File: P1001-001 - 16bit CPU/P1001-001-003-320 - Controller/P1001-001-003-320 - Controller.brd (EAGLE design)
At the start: 200 x 48 mm, 108 parts, among them IC1 74LS138D, IC10 74ALS00D, IC11 74ABT164D, IC12 74ABT164D, IC13 74ABT164D, IC14 74LS138D, IC15 74ABT164D, IC16 74ABT164D, IC17 74ABT164D, IC18 74ABT164D, IC19 74ABT164D, IC2 74LS157D, IC20 74ABT164D, IC3 74LS138D, IC4 74LS138D, IC5 74LS138D, IC6 74LS157D, IC7 74LS157D, IC8 74LS157D, IC9 74LS157D, J1 22-27-2041-04

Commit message: Add the control board
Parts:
- removed ALU_HIGH, ALU_LOW, A_OUT2, B_IN_LOW, B_OUT2, C_REG, RAN_IN_2, STACK: (no value), jumper:JP4
- removed A_CLEAR, B_CLEAR, D_IN, RAM_IN_LOW, X_SWAP: (no value), led:SFH482
- removed BACKBUS, FRONTBUS: (no value), con-harting-ml:ML16
- removed B_IN_HIGH, RAM_PC_OUT, RAN_IN_3: (no value), jumper:JP1
- removed D_REG, RAN_IN_1, X_REG: (no value), jumper:JP2W
- removed IC11, IC12, IC13, IC15, IC16, IC17, IC18, IC19, IC20: 74ABT164D, 74xx-us:SO14
- removed IC14: 74LS138D, 74xx-us:SO16
- removed IC2, IC6, IC7, IC8, IC9: 74LS157D, 74xx-us:SO16
- removed JP5: (no value), jumper:JP2
- removed U$2, U$3: SST39VF1602-70-4I-EKE, 16bit:TSOP48
- added ABC_CLEAR, B_IN_LOW1, HALT_RESEDT_NEXTINS, PC_MAR_IR_IN, RAM_STACK_IN: (no value), jumper:JP2W
- added ADD_HIGH, ADD_LOW, ADD_MID, BA_HIGH, BA_LOW, BB_HIGH, BB_LOW, BC_HIGH, BC_LOW: 74ABT164D, 74xx-us:SO14
- added ADD_SUB, B_IN_HIGH1, CLEAR_OUNS, EXTRA_1_2_PINS, EXTRA_3_4_PINS, EXTRA_5_6_PINS, INTERUPTS, PC_INC_DEC, RAM_IMT_OUT: (no value), jumper:JP1
- added A_CLEAR_LED, B_CLEAR_LED, D_CLEAR_LED, D_HIGH, D_IN_H, D_IN_L, D_LOW, EXTRA1, EXTRA2, EXTRA3, EXTRA4, EXTRA5, EXTRA6, EXTRA_OUT1, EXTRA_OUT2, EXTRA_OUT3, EXTRA_OUT4, INTERUPT_OUT, PAUSE_INERUPT, PC_DEC, PLAY_INTERUPT, RAM_IN_L, ROL, ROR, STEP1, STEP2, STEP3, STEP4: (no value), led:SFH482
- added A_OUT_PINS, B_OUT_PIMS, C_X_OC_STACK_OUT, D_OUT_PINS, EXTRA_OUT, IN_C_D_X, LOGIC_OP, SHIFT_ROLL, STACK_C, STEP_PINS: (no value), jumper:JP4
- added BANKA, BANKB, BANKC: SST39VF1602-70-4I-EKE, 16bit:TSOP48
- added IC21, IC22, IC23: 74LS138D, 74xx-us:SO16
- added IC27: MEGA8535-A, atmel:TQFP44
- added POWER_PINS, READ_WRITE: (no value), jumper:JP2
- added PULL_DOWN, R12, R13, R14: (no value), rcl:M0805
- added R10, R7, R8: (no value), resistor-bourns:SO16
- added RN2: (no value), resistor-dil:SOMC20
- added SV3: (no value), con-harting-ml:ML16
- added SV5: (no value), con-harting-ml:ML6
- added SW_PROD_1, SW_PROD_2, SW_PROD_3, SW_PROD_4, SW_PROD_5: 74LS157D, 74xx-us:SO16
- A_IN_LOW: device jumper:JP4 -> jumper:JP2W
- JP4: device jumper:JP1 -> jumper:JP3Q
- U$1: value SST39VF1602-70-4I-EKE -> 4-DIGIT-7-SEGMENT; device 16bit:TSOP48 -> ADAFRUIT:4-DIGIT-7-SEGMENT
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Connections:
- removed net A-CLEAR: A_CLEAR.K, A_IN_LOW.4, IC14.15
- removed net ADD: ADD.K, ALU_LOW.1, IC3.15
- removed net AND: ALU_HIGH.3, AND.K, IC3.9
- removed net A_HIGH: A_HIGH.K, A_OUT2.2, IC5.14
- removed net A_IN: A_IN.K, A_IN_LOW.3, IC14.14
- removed net A_IN_H_H: A_IN_H_H.K, A_IN_LOW.1, IC14.12
- removed net A_IN_H_L: A_IN_HIGH.1, A_IN_H_L.K, IC14.10
- removed net A_IN_L_H: A_IN_HIGH.2, A_IN_L_H.K, IC14.11
- removed net A_IN_L_L: A_IN_LOW.2, A_IN_L_L.K, IC14.13
- removed net A_LOW: A_LOW.K, A_OUT2.3, IC5.13
- removed net A_OUT: A_OUT.K, A_OUT2.4, IC5.12
- removed net A_SWAP: A_OUT2.1, A_SWAP.K, IC5.15
- removed net BUS0: BACKBUS.1, IC4.1, IC5.1
- removed net BUS1: BACKBUS.2, IC4.2, IC5.2
- removed net BUS10: BACKBUS.11, C_IN.K, C_REG.1
- removed net BUS11: BACKBUS.12, D_IN.K, D_REG.1
- removed net BUS12: BACKBUS.13, X_IN.K, X_REG.1
- removed net BUS13: BACKBUS.14, IR_IN.K, RAN_IN_3.2
- removed net BUS14: BACKBUS.15, MAR_IN.K, RAN_IN_3.1
- removed net BUS15: BACKBUS.16, PC_IN.K, RAN_IN_2.4
- removed net BUS16: FRONTBUS.1, RAM_IN_LOW.K, RAN_IN_2.3
- removed net BUS17: FRONTBUS.2, RAM_IN_H.K, RAN_IN_2.2
- removed net BUS18: FRONTBUS.3, IC3.1
- removed net BUS19: FRONTBUS.4, IC3.2
- removed net BUS2: BACKBUS.3, IC4.3, IC5.3
- removed net BUS20: FRONTBUS.5, IC3.3
- removed net BUS21: FRONTBUS.6, PC_INC.K, RAN_IN_2.1
- removed net BUS22: FRONTBUS.7, STACK.2, STACK_INC.K
- removed net BUS23: FRONTBUS.8, STACK.3, STACK_DEC.K
- removed net BUS24: C_INC.K, C_REG.2, FRONTBUS.9
- removed net BUS25: C_DEC.K, C_REG.3, FRONTBUS.10
- removed net BUS26: FRONTBUS.11, RAN_IN_1.3, RESET.K
- removed net BUS27: FRONTBUS.12, HALT.K, RAN_IN_1.2
- removed net BUS28: FRONTBUS.13, NEXT_INS.K, RAN_IN_1.1
- removed net BUS29: FRONTBUS.14, STACK.1, STACK_IN.K
- removed net BUS3: BACKBUS.4, IC4.4, IC5.4
- removed net BUS30: FRONTBUS.15
- removed net BUS31: FRONTBUS.16
- removed net BUS4: BACKBUS.5, IC14.1
- removed net BUS5: BACKBUS.6, IC14.2
- removed net BUS6: BACKBUS.7, IC14.3
- removed net BUS7: BACKBUS.8, IC1.1
- removed net BUS8: BACKBUS.9, IC1.2
- removed net BUS9: BACKBUS.10, IC1.3
- removed net B_CLEAR: B_CLEAR.K, B_IN_LOW.4, IC1.15
- removed net B_HIGH: B_HIGH.K, B_OUT2.2, IC5.10
- removed net B_IN: B_IN.K, B_IN_LOW.3, IC1.14
- removed net B_IN_H_H: B_IN_H_H.K, B_IN_LOW.1, IC1.12
- removed net B_IN_H_L: B_IN_HIGH.1, B_IN_H_L.K, IC1.10
- removed net B_IN_L_H: B_IN_HIGH.2, B_IN_L_H.K, IC1.11
- removed net B_IN_L_L: B_IN_LOW.2, B_IN_L_L.K, IC1.13
- removed net B_LOW: B_LOW.K, B_OUT2.3, IC5.9
- removed net B_OUT: B_OUT.K, B_OUT2.4, IC5.7
- removed net B_SWAP: B_OUT2.1, B_SWAP.K, IC5.11
- removed net HALT_LED: NEXT_INS.A, R3.13
- removed net NOT: ALU_HIGH.1, IC3.11, NOT.K
- removed net OR: ALU_HIGH.2, IC3.10, OR.K
- removed net PC_OUT: IC4.14, PC_OUT.K
- removed net RAM_OUT: IC4.9, RAM_OUT.K
- removed net SHL: ALU_LOW.3, IC3.13, SHL.K
- removed net SHR: ALU_LOW.4, IC3.12, SHR.K
- removed net SUB: ALU_LOW.2, IC3.14, SUB.K
- removed net XOR: ALU_HIGH.4, IC3.7, XOR.K
- new net A: IC27.37, RN2.20
- new net B: IC27.36, RN2.19
- new net BANKA_PROG: BANKA.11, JP4.5, R12.1
- new net BANKB_PROG: BANKB.11, JP4.3, R13.1
- new net BANKC_PROG: BANKC.11, JP4.1, R14.1
- new net C: IC27.35, RN2.18
- new net D: IC27.34, RN2.17
- new net DIG0: IC27.40, U$1.PIN14
- new net DIG1: IC27.41, U$1.PIN11
- new net DIG2: IC27.42, U$1.PIN10
- new net DIG3: IC27.43, U$1.PIN6
- new net DP: IC27.30, RN2.13
- new net E: IC27.33, RN2.16
- new net EXTERN_BUS0: IC27.9, R10.1, SV3.1
- new net EXTERN_BUS1: IC27.10, R10.9, SV3.2
- new net EXTERN_BUS10: IC27.21, R10.6, SV3.11
- new net EXTERN_BUS11: IC27.22, R10.14, SV3.12
- new net EXTERN_BUS12: IC27.23, R10.7, SV3.13
- new net EXTERN_BUS13: IC27.24, R10.15, SV3.14
- new net EXTERN_BUS14: IC27.25, R10.8, SV3.15
- new net EXTERN_BUS15: IC27.26, PULL_DOWN.1, SV3.16
- new net EXTERN_BUS2: IC27.11, R10.2, SV3.3
- new net EXTERN_BUS3: IC27.12, R10.10, SV3.4
- new net EXTERN_BUS4: IC27.13, R10.3, SV3.5
- new net EXTERN_BUS5: IC27.14, R10.11, SV3.6
- new net EXTERN_BUS6: IC27.15, R10.4, SV3.7
- new net EXTERN_BUS7: IC27.16, R10.12, SV3.8
- new net EXTERN_BUS8: IC27.19, R10.5, SV3.9
- new net EXTERN_BUS9: IC27.20, R10.13, SV3.10
- new net F: IC27.32, RN2.15
- new net G: IC27.31, RN2.14
- new net N$100: D_OUT.A, R3.14
- new net N$101: D_LOW.A, R3.13
- new net N$102: D_HIGH.A, R3.12
- new net N$103: D_SWAP.A, R3.11
- new net N$104: R3.10, X_OUT.A
- new net N$105: PC_OUT.A, R3.9
- new net N$106: IC5.15, RAM_IMT_OUT.1, RAM_OUT.K
- new net N$107: IC5.14, INTERUPT_OUT.K, RAM_IMT_OUT.2
- new net N$108: EXTRA_OUT.4, EXTRA_OUT1.K, IC5.13
- new net N$109: EXTRA_OUT.3, EXTRA_OUT2.K, IC5.12
- new net N$110: EXTRA_OUT.2, EXTRA_OUT3.K, IC5.11
- new net N$111: EXTRA_OUT.1, EXTRA_OUT4.K, IC5.10
- new net N$112: R2.1, STACK_OUT.A
- new net N$113: EXTRA_OUT4.A, R2.8
- new net N$114: EXTRA_OUT3.A, R2.7
- new net N$115: EXTRA_OUT2.A, R2.6
- new net N$116: EXTRA_OUT1.A, R2.5
- new net N$117: R2.2, RAM_OUT.A
- new net N$118: INTERUPT_OUT.A, R2.3
- new net N$119: IC27.1, SV5.3
- new net N$120: IC27.3, SV5.4
- new net N$121: IC27.2, SV5.6
- new net N$122: IC27.4, SV5.2
- new net N$123: RN2.1, U$1.PIN13
- new net N$124: RN2.2, U$1.PIN9
- new net N$125: RN2.3, U$1.PIN4
- new net N$126: RN2.4, U$1.PIN2
- new net N$127: RN2.5, U$1.PIN1
- new net N$128: RN2.6, U$1.PIN12
- new net N$129: RN2.7, U$1.PIN5
- new net N$130: RN2.8, U$1.PIN3
- new net N$131: R2.15, STEP1.A
- new net N$132: R2.14, STEP2.A
- new net N$133: R2.13, STEP3.A
- new net N$134: R2.12, STEP4.A
- new net N$37: BANKA.27, BANKA.46, BANKB.27, BANKB.46, BANKC.27, BANKC.46
- new net N$42: BANKA.28, BANKB.28, BANKC.28, READ_WRITE.2
- new net N$43: EXTRA5.A, R8.5
- new net N$63: IC1.13, SHIFT_ROLL.4, SHL.K
- new net N$64: IC1.12, SHIFT_ROLL.3, SHR.K
- new net N$65: IC1.11, ROL.K, SHIFT_ROLL.2
- new net N$66: IC1.10, ROR.K, SHIFT_ROLL.1
- new net N$67: NOT.A, R7.9
- new net N$68: AND.A, R7.10
- new net N$69: OR.A, R7.11
- new net N$70: R7.12, XOR.A
- new net N$71: IC23.7, LOGIC_OP.1, XOR.K
- new net N$72: IC23.9, LOGIC_OP.2, OR.K
- new net N$73: AND.K, IC23.10, LOGIC_OP.3
- new net N$74: IC23.11, LOGIC_OP.4, NOT.K
- new net N$75: A_OUT.K, A_OUT_PINS.1, IC3.15
- new net N$76: A_LOW.K, A_OUT_PINS.2, IC3.14
- new net N$77: A_HIGH.K, A_OUT_PINS.3, IC3.13
- new net N$78: A_OUT_PINS.4, A_SWAP.K, IC3.12
- new net N$79: B_OUT.K, B_OUT_PIMS.1, IC3.11
- new net N$80: B_LOW.K, B_OUT_PIMS.2, IC3.10
- new net N$81: B_HIGH.K, B_OUT_PIMS.3, IC3.9
- new net N$82: B_OUT_PIMS.4, B_SWAP.K, IC3.7
- new net N$83: D_OUT.K, D_OUT_PINS.1, IC4.14
- new net N$84: C_OUT.K, C_X_OC_STACK_OUT.4, IC4.15
- new net N$85: D_LOW.K, D_OUT_PINS.2, IC4.13
- new net N$86: D_HIGH.K, D_OUT_PINS.3, IC4.12
- new net N$87: D_OUT_PINS.4, D_SWAP.K, IC4.11
- new net N$88: C_X_OC_STACK_OUT.3, IC4.10, X_OUT.K
- new net N$89: C_X_OC_STACK_OUT.2, IC4.9, PC_OUT.K
- new net N$90: C_X_OC_STACK_OUT.1, IC4.7, STACK_OUT.K
- new net N$91: A_OUT.A, R3.1
- new net N$92: A_LOW.A, R3.2
- new net N$93: A_HIGH.A, R3.3
- new net N$94: A_SWAP.A, R3.4
- new net N$95: B_OUT.A, R3.5
- new net N$96: B_LOW.A, R3.6
- new net N$97: B_HIGH.A, R3.7
- new net N$98: B_SWAP.A, R3.8
- new net N$99: C_OUT.A, R3.15
- new net WRITE_ENABLE: BANKA.14, BANKB.14, BANKC.14, JP3.2
- net !CLEAR: now also BANKA.12, BANKB.12, BANKC.12, CLEAR_OUNS.1; no longer JP4.1
- net ADDR_BUS0: now also BANKA.25, BANKB.25, BANKC.25, SW_PROD_1.12; no longer IC7.12, U$1.25, U$2.25, U$3.25
- net ADDR_BUS1: now also BANKA.24, BANKB.24, BANKC.24, SW_PROD_1.9; no longer IC7.9, U$1.24, U$2.24, U$3.24
- net ADDR_BUS10: now also BANKA.6, BANKB.6, BANKC.6, SW_PROD_3.7; no longer IC2.7, U$1.6, U$2.6, U$3.6
- net ADDR_BUS11: now also BANKA.5, BANKB.5, BANKC.5, SW_PROD_3.4; no longer IC2.4, U$1.5, U$2.5, U$3.5
- net ADDR_BUS12: now also BANKA.4, BANKB.4, BANKC.4, SW_PROD_4.4; no longer IC8.4, U$1.4, U$2.4, U$3.4
- net ADDR_BUS13: now also BANKA.3, BANKB.3, BANKC.3, SW_PROD_4.7; no longer IC8.7, U$1.3, U$2.3, U$3.3
- net ADDR_BUS14: now also BANKA.2, BANKB.2, BANKC.2, SW_PROD_4.9; no longer IC8.9, U$1.2, U$2.2, U$3.2
- net ADDR_BUS15: now also BANKA.1, BANKB.1, BANKC.1, SW_PROD_4.12; no longer IC8.12, U$1.1, U$2.1, U$3.1
- net ADDR_BUS16: now also BANKA.48, BANKB.48, BANKC.48, SW_PROD_5.4; no longer IC9.4, U$1.48, U$2.48, U$3.48
- net ADDR_BUS17: now also BANKA.17, BANKB.17, BANKC.17, SW_PROD_5.7; no longer IC9.7, U$1.17, U$2.17, U$3.17
- net ADDR_BUS18: now also BANKA.16, BANKB.16, BANKC.16, SW_PROD_5.9; no longer IC9.9, U$1.16, U$2.16, U$3.16
- net ADDR_BUS19: now also BANKA.9, BANKB.9, BANKC.9, SW_PROD_5.12; no longer IC9.12, U$1.9, U$2.9, U$3.9
- net ADDR_BUS2: now also BANKA.23, BANKB.23, BANKC.23, SW_PROD_1.7; no longer IC7.7, U$1.23, U$2.23, U$3.23
- net ADDR_BUS3: now also BANKA.22, BANKB.22, BANKC.22, SW_PROD_1.4; no longer IC7.4, U$1.22, U$2.22, U$3.22
- net ADDR_BUS4: now also BANKA.21, BANKB.21, BANKC.21, SW_PROD_2.12; no longer IC6.12, U$1.21, U$2.21, U$3.21
- net ADDR_BUS5: now also BANKA.20, BANKB.20, BANKC.20, SW_PROD_2.9; no longer IC6.9, U$1.20, U$2.20, U$3.20
- net ADDR_BUS6: now also BANKA.19, BANKB.19, BANKC.19, SW_PROD_2.7; no longer IC6.7, U$1.19, U$2.19, U$3.19
- net ADDR_BUS7: now also BANKA.18, BANKB.18, BANKC.18, SW_PROD_2.4; no longer IC6.4, U$1.18, U$2.18, U$3.18
- net ADDR_BUS8: now also BANKA.8, BANKB.8, BANKC.8, SW_PROD_3.12; no longer IC2.12, U$1.8, U$2.8, U$3.8
- net ADDR_BUS9: now also BANKA.7, BANKB.7, BANKC.7, SW_PROD_3.9; no longer IC2.9, U$1.7, U$2.7, U$3.7
- net ADDR_SHIFT: now also ADD_LOW.1, ADD_LOW.2; no longer IC11.1, IC11.2
- net CLEAR: now also CLEAR_OUNS.2; no longer JP4.2
- net CLK: now also POWER_PINS.1; no longer JP5.1
- net DATAA0: now also BANKA.29, BA_LOW.3, IC3.1, IC4.1, IC5.1; no longer IC15.3, U$1.29
- net DATAA1: now also BANKA.31, BA_LOW.4, IC3.2, IC4.2, IC5.2; no longer IC15.4, U$1.31
- net DATAA10: now also BANKA.34, BA_HIGH.5, EXTRA6.K, EXTRA_5_6_PINS.2; no longer IC16.5, U$1.34
- net DATAA11: now also ABC_CLEAR.1, A_CLEAR_LED.K, BANKA.36, BA_HIGH.6; no longer IC16.6, U$1.36
- net DATAA12: now also ABC_CLEAR.2, BANKA.39, BA_HIGH.10, B_CLEAR_LED.K; no longer IC16.10, U$1.39
- net DATAA13: now also ABC_CLEAR.3, BANKA.41, BA_HIGH.11, D_CLEAR_LED.K; no longer IC16.11, U$1.41
- net DATAA14: now also BANKA.43, BA_HIGH.12, INTERUPTS.1, PAUSE_INERUPT.K; no longer IC16.12, U$1.43
- net DATAA15: now also BANKA.45, BA_HIGH.13, INTERUPTS.2, PLAY_INTERUPT.K; no longer IC16.13, U$1.45
- net DATAA2: now also BANKA.33, BA_LOW.5, IC3.3, IC4.3, IC5.3; no longer IC15.5, U$1.33
- net DATAA3: now also BANKA.35, BA_LOW.6, IC3.4, IC4.4, IC5.4; no longer IC15.6, U$1.35
- net DATAA4: now also BANKA.38, BA_LOW.10, IC3.5, IC4.5, IC5.5; no longer IC15.10, U$1.38
- net DATAA5: now also BANKA.40, BA_LOW.11, EXTRA1.K, EXTRA_1_2_PINS.1; no longer IC15.11, U$1.40
- net DATAA6: now also BANKA.42, BA_LOW.12, EXTRA2.K, EXTRA_1_2_PINS.2; no longer IC15.12, U$1.42
- net DATAA7: now also BANKA.44, BA_HIGH.1, BA_HIGH.2, BA_LOW.13, EXTRA3.K, EXTRA_3_4_PINS.1; no longer IC15.13, IC16.1, IC16.2, U$1.44
- net DATAA8: now also BANKA.30, BA_HIGH.3, EXTRA4.K, EXTRA_3_4_PINS.2; no longer IC16.3, U$1.30
- net DATAA9: now also BANKA.32, BA_HIGH.4, EXTRA5.K, EXTRA_5_6_PINS.1; no longer IC16.4, U$1.32
- net DATAA_SHIFT: now also BA_LOW.1, BA_LOW.2; no longer IC15.1, IC15.2
- net DATAB0: now also BANKB.29, BB_LOW.3, IC21.1; no longer IC17.3, U$2.29
- net DATAB1: now also BANKB.31, BB_LOW.4, IC21.2; no longer IC17.4, U$2.31
- net DATAB10: now also BANKB.34, BB_HIGH.5, IR_IN.K, PC_MAR_IR_IN.1; no longer IC18.5, U$2.34
- net DATAB11: now also BANKB.36, BB_HIGH.6, MAR_IN.K, PC_MAR_IR_IN.2; no longer IC18.6, U$2.36
- net DATAB12: now also BANKB.39, BB_HIGH.10, PC_IN.K, PC_MAR_IR_IN.3; no longer IC18.10, U$2.39
- net DATAB13: now also BANKB.41, BB_HIGH.11, RAM_STACK_IN.1, STACK_IN.K; no longer IC18.11, U$2.41
- net DATAB14: now also BANKB.43, BB_HIGH.12, RAM_IN_L.K, RAM_STACK_IN.2; no longer IC18.12, U$2.43
- net DATAB15: now also BANKB.45, BB_HIGH.13, RAM_IN_H.K, RAM_STACK_IN.3; no longer IC18.13, U$2.45
- net DATAB2: now also BANKB.33, BB_LOW.5, IC21.3; no longer IC17.5, U$2.33
- net DATAB3: now also BANKB.35, BB_LOW.6, IC22.1; no longer IC17.6, U$2.35
- net DATAB4: now also BANKB.38, BB_LOW.10, IC22.2, PC_INC_DEC.2; no longer IC17.10, U$2.38
- net DATAB5: now also BANKB.40, BB_LOW.11, IC22.3; no longer IC17.11, U$2.40
- net DATAB6: now also BANKB.42, BB_LOW.12, C_IN.K, IN_C_D_X.1; no longer IC17.12, U$2.42
- net DATAB7: now also BANKB.44, BB_HIGH.1, BB_HIGH.2, BB_LOW.13, D_IN_L.K, IN_C_D_X.2; no longer IC17.13, IC18.1, IC18.2, U$2.44
- net DATAB8: now also BANKB.30, BB_HIGH.3, D_IN_H.K, IN_C_D_X.3; no longer IC18.3, U$2.30
- net DATAB9: now also BANKB.32, BB_HIGH.4, IN_C_D_X.4, X_IN.K; no longer IC18.4, U$2.32
- net DATAB_SHIFT: now also BB_LOW.1, BB_LOW.2; no longer IC17.1, IC17.2
- net DATAC0: now also BANKC.29, BC_LOW.3, IC1.1, IC23.1; no longer IC19.3, U$3.29
- net DATAC1: now also BANKC.31, BC_LOW.4, IC1.2, IC23.2; no longer IC19.4, U$3.31
- net DATAC10: now also BANKC.34, BC_HIGH.5; no longer IC20.5, U$3.34
- net DATAC11: now also BANKC.36, BC_HIGH.6; no longer IC20.6, U$3.36
- net DATAC12: now also BANKC.39, BC_HIGH.10; no longer IC20.10, U$3.39
- net DATAC13: now also BANKC.41, BC_HIGH.11, HALT_RESEDT_NEXTINS.3, RESET.K; no longer IC20.11, U$3.41
- net DATAC14: now also BANKC.43, BC_HIGH.12, HALT.K, HALT_RESEDT_NEXTINS.2; no longer IC20.12, U$3.43
- net DATAC15: now also BANKC.45, BC_HIGH.13, HALT_RESEDT_NEXTINS.1, NEXT_INS.K; no longer IC20.13, U$3.45
- net DATAC2: now also BANKC.33, BC_LOW.5, IC1.3, IC23.3; no longer IC19.5, U$3.33
- net DATAC3: now also BANKC.35, BC_LOW.6, IC1.4, IC23.4; no longer IC19.6, U$3.35
- net DATAC4: now also BANKC.38, BC_LOW.10, PC_DEC.K; no longer IC19.10, U$3.38
- net DATAC5: now also BANKC.40, BC_LOW.11, PC_INC.K, PC_INC_DEC.1; no longer IC19.11, U$3.40
- net DATAC6: now also BANKC.42, BC_LOW.12, STACK_C.4, STACK_INC.K; no longer IC19.12, U$3.42
- net DATAC7: now also BANKC.44, BC_HIGH.1, BC_HIGH.2, BC_LOW.13, STACK_C.3, STACK_DEC.K; no longer IC19.13, IC20.1, IC20.2, U$3.44
- net DATAC8: now also BANKC.30, BC_HIGH.3, C_INC.K, STACK_C.2; no longer IC20.3, U$3.30
- net DATAC9: now also BANKC.32, BC_HIGH.4, C_DEC.K, STACK_C.1; no longer IC20.4, U$3.32
- net DATAC_SHIFT: now also BC_LOW.1, BC_LOW.2; no longer IC19.1, IC19.2
- net DATA_ADDR_CLOCK: now also BA_HIGH.8, BA_LOW.8, BB_HIGH.8, BB_LOW.8, BC_HIGH.8, BC_LOW.8; no longer IC15.8, IC16.8, IC17.8, IC18.8, IC19.8, IC20.8
- net GND: now also ADD_HIGH.7, ADD_LOW.7, ADD_MID.7, BANKA.26, BANKA.37, BANKB.26, BANKB.37, BANKC.26, BANKC.37, BA_HIGH.7, BA_LOW.7, BB_HIGH.7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; no longer IC1.4, IC11.7, IC12.7, IC13.7, IC14.4, IC14.5, IC14.8, IC15.7, IC16.7, IC17.7, IC18.7, IC19.7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
- net IN_BUS0: now also STEP1.K, STEP_PINS.1, SW_PROD_1.14; no longer IC7.14
- net IN_BUS1: now also STEP2.K, STEP_PINS.2, SW_PROD_1.11; no longer IC7.11
- net IN_BUS10: now also SW_PROD_3.5; no longer IC2.5
- net IN_BUS11: now also SW_PROD_3.2; no longer IC2.2
- net IN_BUS12: now also SW_PROD_4.2; no longer IC8.2
- net IN_BUS13: now also SW_PROD_4.5; no longer IC8.5
- net IN_BUS14: now also SW_PROD_4.11; no longer IC8.11
- net IN_BUS15: now also SW_PROD_4.14; no longer IC8.14
- net IN_BUS16: now also SW_PROD_5.2; no longer IC9.2
- net IN_BUS17: now also SW_PROD_5.5; no longer IC9.5
- net IN_BUS18: now also SW_PROD_5.11; no longer IC9.11
- net IN_BUS19: now also SW_PROD_5.14; no longer IC9.14
- net IN_BUS2: now also STEP3.K, STEP_PINS.3, SW_PROD_1.5; no longer IC7.5
- net IN_BUS3: now also STEP4.K, STEP_PINS.4, SW_PROD_1.2; no longer IC7.2
- net IN_BUS4: now also SW_PROD_2.14; no longer IC6.14
- net IN_BUS5: now also SW_PROD_2.11; no longer IC6.11
- net IN_BUS6: now also SW_PROD_2.5; no longer IC6.5
- net IN_BUS7: now also SW_PROD_2.2; no longer IC6.2
- net IN_BUS8: now also SW_PROD_3.14; no longer IC2.14
- net IN_BUS9: now also SW_PROD_3.11; no longer IC2.11
- net N$10: now also D_CLEAR_LED.A, R8.9; no longer IC4.11, X_REG.2, X_SWAP.K
- net N$11: now also PAUSE_INERUPT.A, R8.10; no longer R3.2, X_IN.A
- net N$12: now also PLAY_INTERUPT.A, R8.11; no longer IC4.7, X_OUT.K, X_REG.3
- net N$13: now also C_IN.A, R8.12; no longer R3.15, X_OUT.A
- net N$14: now also D_IN_L.A, R8.15; no longer R3.9, STACK_IN.A
- net N$15: now also D_IN_H.A, R8.14; no longer R3.10, STACK_INC.A
- net N$16: now also PC_INC.A, R5.1; no longer R3.11, STACK_DEC.A
- net N$17: now also PC_DEC.A, R5.2; no longer R3.12, STACK_OUT.A
- net N$18: now also IR_IN.A, R5.3; no longer IC4.13, STACK.4, STACK_OUT.K
- net N$19: now also MAR_IN.A, R5.4; no longer D_REG.2, D_SWAP.K, IC4.15
- net N$2: now also EXTRA1.A, R8.1; no longer C_IN.A, R3.8
- net N$20: now also PC_IN.A, R5.5; no longer D_SWAP.A, R3.14
- net N$21: now also R5.6, STACK_IN.A; no longer A_CLEAR.A, R5.9
- net N$22: now also R5.7, RAM_IN_L.A; no longer ADD.A, R5.1
- net N$23: now also R5.8, RAM_IN_H.A; no longer A_IN.A, R5.10
- net N$24: now also NEXT_INS.A, R5.10; no longer B_CLEAR.A, R4.9
- net N$25: now also R5.15, STACK_DEC.A; no longer B_IN.A, R4.10
- net N$26: now also C_INC.A, R5.14; no longer B_IN_L_L.A, R4.11
- net N$27: now also C_DEC.A, R5.13; no longer B_IN_H_H.A, R4.12
- net N$28: now also R5.12, RESET.A; no longer R5.8, XOR.A
- net N$29: now also HALT.A, R5.11; no longer AND.A, R5.7
- net N$3: now also EXTRA2.A, R8.2; no longer C_OUT.K, C_REG.4, IC4.10
- net N$30: now also R5.9, STACK_INC.A; no longer OR.A, R5.6
- net N$31: now also A_IN.K, A_IN_LOW.1, IC21.15; no longer NOT.A, R5.5
- net N$32: now also A_IN_LOW.2, A_IN_L_L.K, IC21.14; no longer R5.4, SHR.A
- net N$33: now also A_IN_H_H.K, A_IN_LOW.3, IC21.13; no longer R5.3, SHL.A
- net N$34: now also A_IN_HIGH.1, A_IN_L_H.K, IC21.12; no longer R5.2, SUB.A
- net N$35: now also A_IN_HIGH.2, A_IN_H_L.K, IC21.11; no longer B_IN_L_H.A, R4.13
- net N$36: now also A_IN.A, R4.8; no longer B_IN_H_L.A, R4.14
- net N$38: now also R4.7; no longer R5.11
- net N$39: now also R4.6; no longer R5.12
- net N$4: now also R8.13, X_IN.A; no longer C_OUT.A, R3.5
- net N$40: now also R4.5; no longer R5.13
- net N$41: now also R4.4; no longer R5.14
- net N$44: now also B_IN.A, B_IN_LOW1.3, IC22.15; no longer R2.15, RAM_OUT.A, RAM_PC_OUT.2
- net N$45: now also B_IN_LOW1.2, B_IN_L_L.A, IC22.14; no longer A_SWAP.A, R2.1
- net N$46: now also B_IN_H_H.A, B_IN_LOW1.1, IC22.13; no longer A_HIGH.A, R2.2
- net N$47: now also B_IN_HIGH1.2, B_IN_L_H.A, IC22.12; no longer A_LOW.A, R2.3
- net N$48: now also B_IN_HIGH1.1, B_IN_H_L.A, IC22.11; no longer A_OUT.A, R2.4
- net N$49: now also B_IN.K, R4.9; no longer B_SWAP.A, R2.5
- net N$5: now also EXTRA4.A, R8.4; no longer C_DEC.A, R3.6
- net N$51: now also B_IN_L_L.K, R4.10; no longer B_HIGH.A, R2.6
- net N$52: now also B_IN_H_H.K, R4.11; no longer B_LOW.A, R2.7
- net N$53: now also B_IN_L_H.K, R4.12; no longer B_OUT.A, R2.8
- net N$54: now also B_IN_H_L.K, R4.14; no longer PC_OUT.A, R2.14, RAM_PC_OUT.1
- net N$55: now also R7.8, ROR.A; no longer IR_IN.A, R4.8
- net N$56: now also R7.7, ROL.A; no longer MAR_IN.A, R4.7
- net N$57: now also R7.6, SHR.A; no longer PC_IN.A, R4.6
- net N$58: now also R7.5, SHL.A; no longer R4.5, RAM_IN_LOW.A
- net N$59: now also R7.4, SUB.A; no longer R4.4, RAM_IN_H.A
- net N$6: now also EXTRA3.A, R8.3; no longer C_INC.A, R3.7
- net N$60: now also ADD.A, R7.3; no longer PC_INC.A, R4.3
- net N$61: now also ADD.K, ADD_SUB.2, IC1.15; no longer R4.2, RESET.A
- net N$62: now also ADD_SUB.1, IC1.14, SUB.K; no longer HALT.A, R4.1
- net N$7: now also EXTRA6.A, R8.6; no longer D_OUT.A, D_OUT.K, D_REG.3, IC4.12, R3.3
- net N$8: now also B_CLEAR_LED.A, R8.8; no longer D_IN.A, R3.4
- net N$9: now also A_CLEAR_LED.A, R8.7; no longer R3.1, X_SWAP.A
- net PROGRAM: now also JP4.2, JP4.4, JP4.6
- net PROG_ADDR0: now also ADD_LOW.3, SW_PROD_1.13; no longer IC11.3, IC7.13
- net PROG_ADDR1: now also ADD_LOW.4, SW_PROD_1.10; no longer IC11.4, IC7.10
- net PROG_ADDR10: now also ADD_MID.5, SW_PROD_3.6; no longer IC12.5, IC2.6
- net PROG_ADDR11: now also ADD_MID.6, SW_PROD_3.3; no longer IC12.6, IC2.3
- net PROG_ADDR12: now also ADD_MID.10, SW_PROD_4.3; no longer IC12.10, IC8.3
- net PROG_ADDR13: now also ADD_MID.11, SW_PROD_4.6; no longer IC12.11, IC8.6
- net PROG_ADDR14: now also ADD_MID.12, SW_PROD_4.10; no longer IC12.12, IC8.10
- net PROG_ADDR15: now also ADD_HIGH.1, ADD_HIGH.2, ADD_MID.13, SW_PROD_4.13; no longer IC12.13, IC13.1, IC13.2, IC8.13
- net PROG_ADDR16: now also ADD_HIGH.3, SW_PROD_5.3; no longer IC13.3, IC9.3
- net PROG_ADDR17: now also ADD_HIGH.4, SW_PROD_5.6; no longer IC13.4, IC9.6
- net PROG_ADDR18: now also ADD_HIGH.5, SW_PROD_5.10; no longer IC13.5, IC9.10
- net PROG_ADDR19: now also ADD_HIGH.6, SW_PROD_5.13; no longer IC13.6, IC9.13
- net PROG_ADDR2: now also ADD_LOW.5, SW_PROD_1.6; no longer IC11.5, IC7.6
- net PROG_ADDR3: now also ADD_LOW.6, SW_PROD_1.3; no longer IC11.6, IC7.3
- net PROG_ADDR4: now also ADD_LOW.10, SW_PROD_2.13; no longer IC11.10, IC6.13
- net PROG_ADDR5: now also ADD_LOW.11, SW_PROD_2.10; no longer IC11.11, IC6.10
- net PROG_ADDR6: now also ADD_LOW.12, SW_PROD_2.6; no longer IC11.12, IC6.6
- net PROG_ADDR7: now also ADD_LOW.13, ADD_MID.1, ADD_MID.2, SW_PROD_2.3; no longer IC11.13, IC12.1, IC12.2, IC6.3
- net PROG_ADDR8: now also ADD_MID.3, SW_PROD_3.13; no longer IC12.3, IC2.13
- net PROG_ADDR9: now also ADD_MID.4, SW_PROD_3.10; no longer IC12.4, IC2.10
- net PROG_ADDR_CLOCK: now also ADD_HIGH.8, ADD_LOW.8, ADD_MID.8; no longer IC11.8, IC12.8, IC13.8
- net PROG_CLEAR: now also ADD_HIGH.9, ADD_LOW.9, ADD_MID.9, BA_HIGH.9, BA_LOW.9, BB_HIGH.9, BB_LOW.9, BC_HIGH.9, BC_LOW.9; no longer IC11.9, IC12.9, IC13.9, IC15.9, IC16.9, IC17.9, IC18.9, IC19.9, IC20.9
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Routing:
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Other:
- board size 200 x 48 mm -> 200 x 152 mm

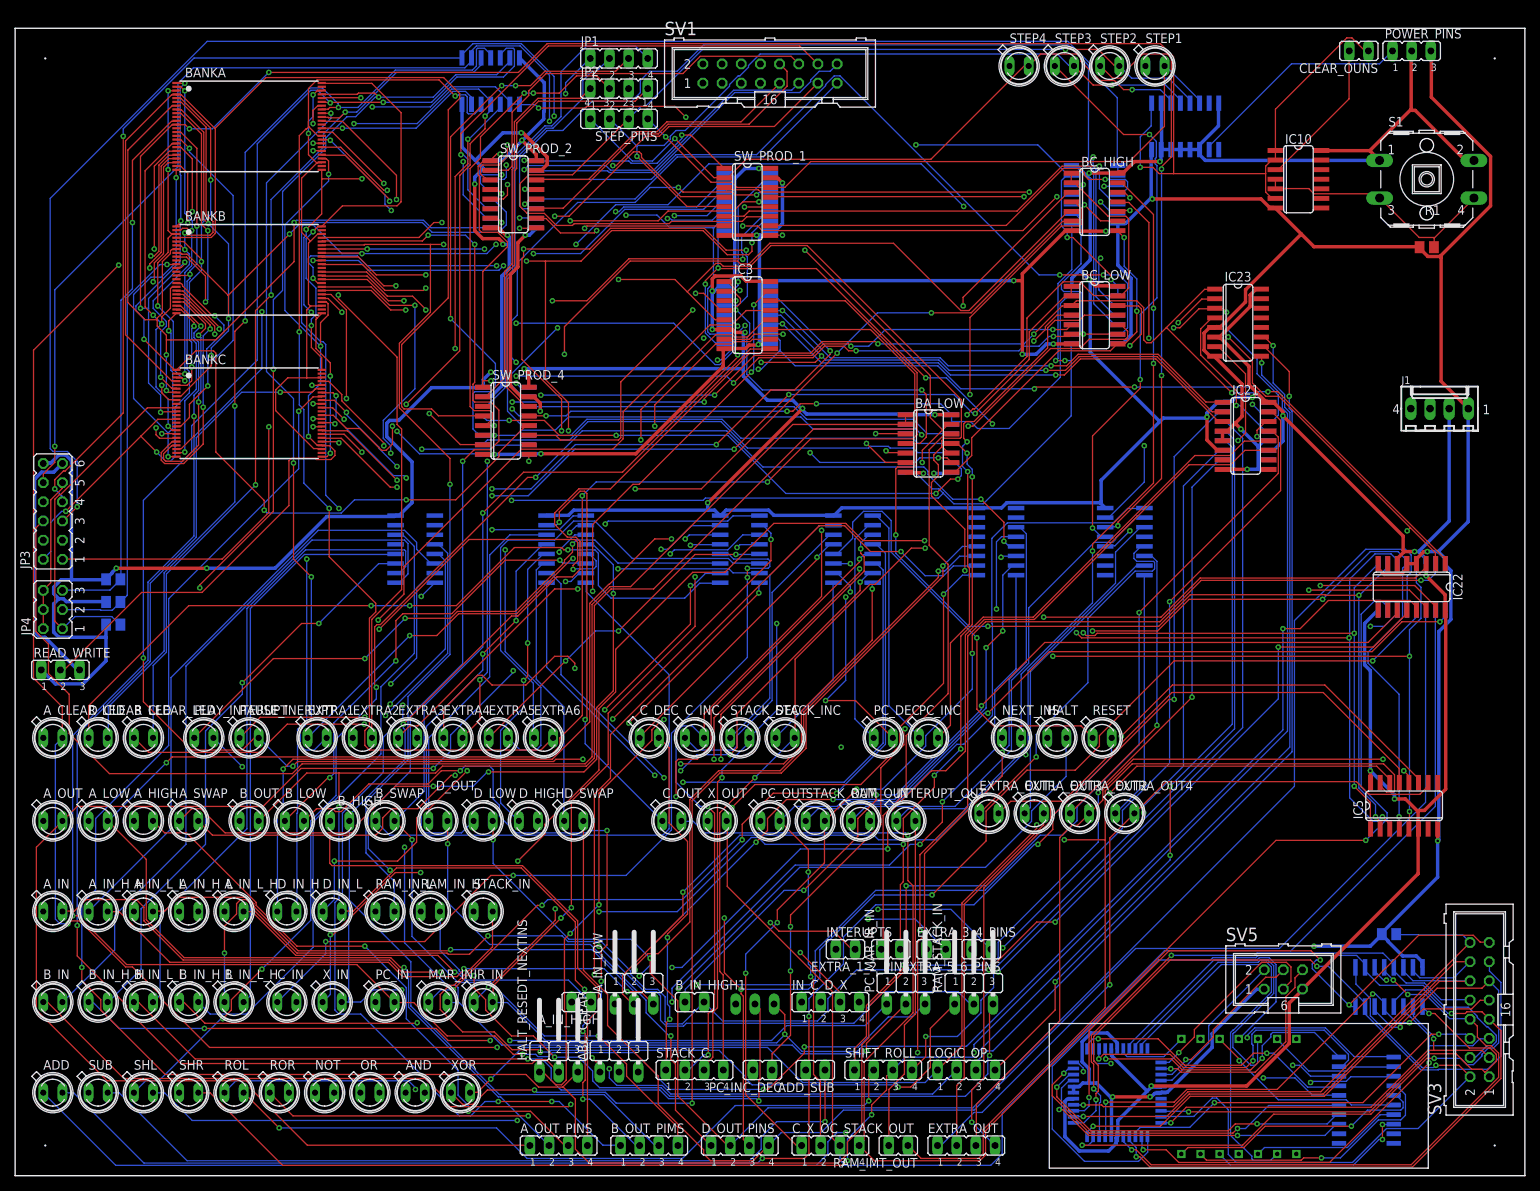
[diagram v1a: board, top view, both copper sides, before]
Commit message: Controller done?
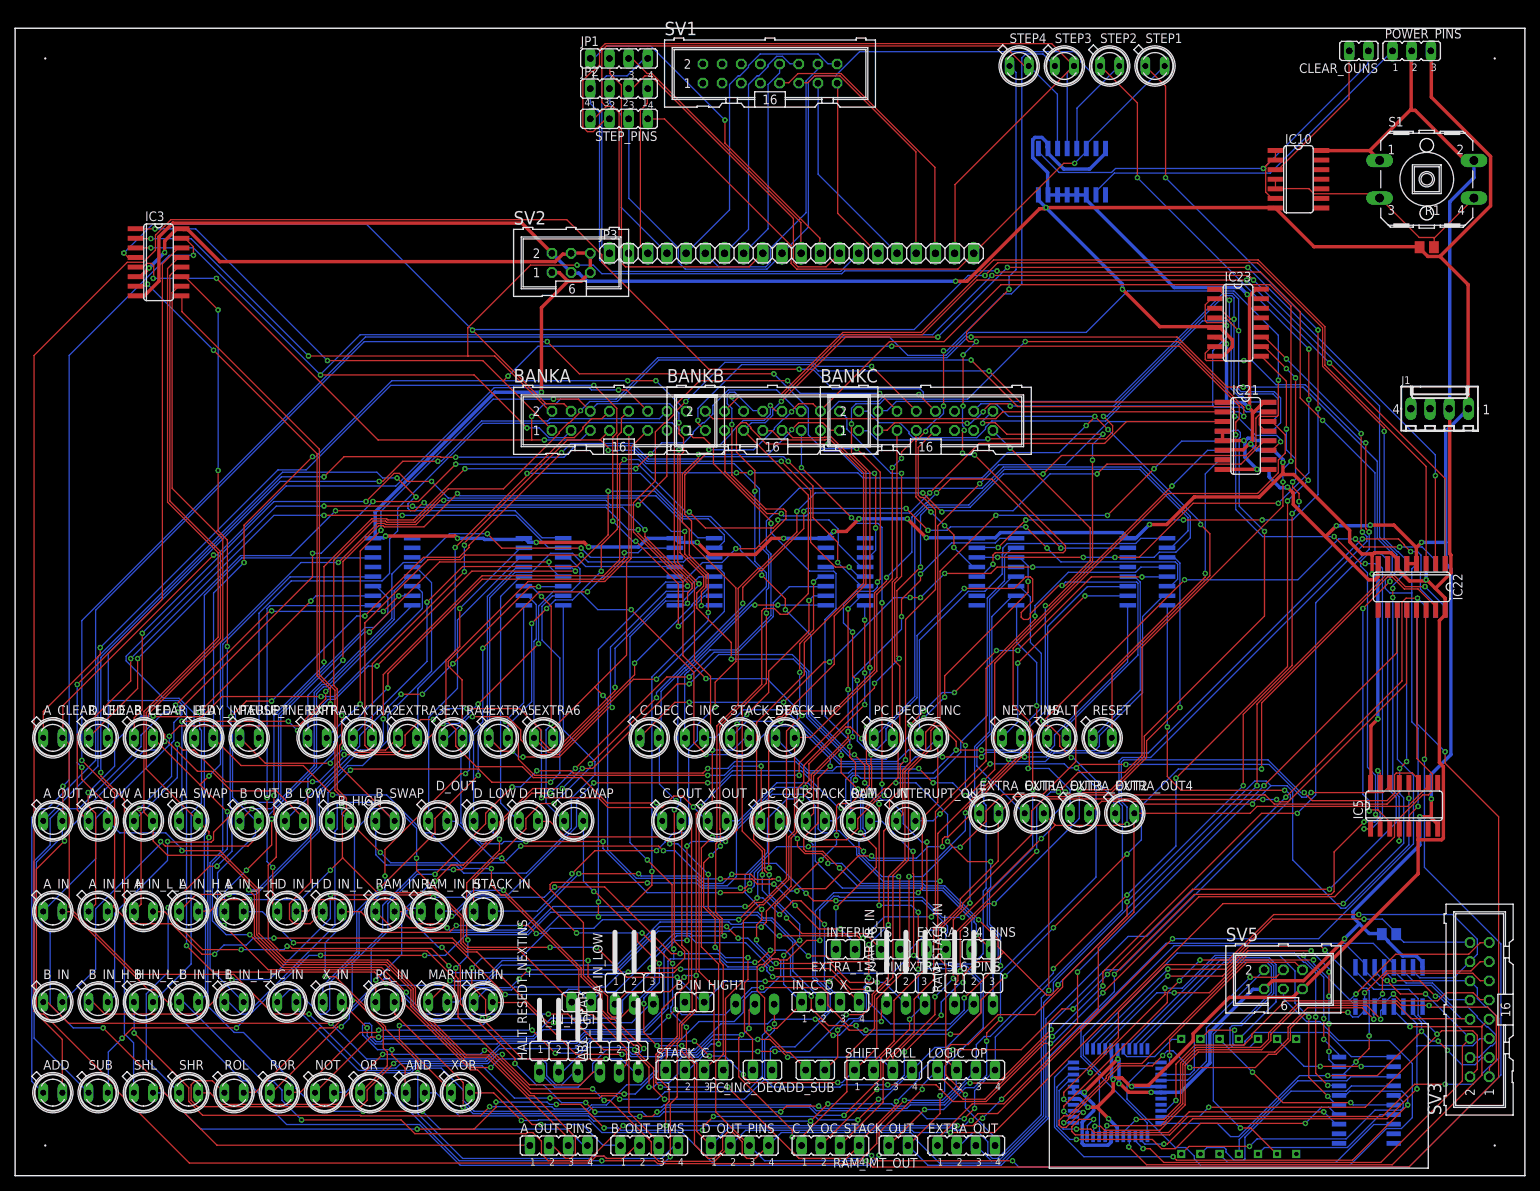
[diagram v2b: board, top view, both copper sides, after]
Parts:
- removed ADD_HIGH, ADD_LOW, ADD_MID, BA_HIGH, BA_LOW, BB_HIGH, BB_LOW, BC_HIGH, BC_LOW: 74ABT164D, 74xx-us:SO14
- removed JP4: (no value), jumper:JP3Q
- removed R12, R13, R14: (no value), rcl:M0805
- removed READ_WRITE: (no value), jumper:JP2
- removed SW_PROD_1, SW_PROD_2, SW_PROD_3, SW_PROD_4, SW_PROD_5: 74LS157D, 74xx-us:SO16
- added SV2: (no value), con-harting-ml:ML6
- BANKA, BANKB, BANKC: value SST39VF1602-70-4I-EKE -> (none); device 16bit:TSOP48 -> con-harting-ml:ML16
- JP3: device jumper:JP6Q -> pinhead:1X20
- moved JP3 103.7 mm to (102.9, 122.2), turned to 0 degrees
- moved BANKC 89.6 mm to (120.6, 100.0)
- moved IC3 78.3 mm to (19.0, 121.0)
- moved BANKB 72.1 mm to (100.3, 100.0)
- moved BANKA 62.6 mm to (80.0, 100.0)
- moved R5 39.1 mm to (150.0, 80.0)
- moved R7 20.4 mm to (110.0, 80.0)
- moved R2 17.5 mm to (130.0, 80.0)
- moved U$4 16.2 mm to (140.0, 133.0)
- moved R8 6.71 mm to (90.0, 80.0)
- moved R3 4.24 mm to (70.0, 80.0)
- moved R4 4.24 mm to (50.0, 80.0)
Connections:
- removed net ADDR_BUS0: BANKA.25, BANKB.25, BANKC.25, SW_PROD_1.12
- removed net ADDR_BUS1: BANKA.24, BANKB.24, BANKC.24, SW_PROD_1.9
- removed net ADDR_BUS10: BANKA.6, BANKB.6, BANKC.6, SW_PROD_3.7
- removed net ADDR_BUS11: BANKA.5, BANKB.5, BANKC.5, SW_PROD_3.4
- removed net ADDR_BUS12: BANKA.4, BANKB.4, BANKC.4, SW_PROD_4.4
- removed net ADDR_BUS13: BANKA.3, BANKB.3, BANKC.3, SW_PROD_4.7
- removed net ADDR_BUS14: BANKA.2, BANKB.2, BANKC.2, SW_PROD_4.9
- removed net ADDR_BUS15: BANKA.1, BANKB.1, BANKC.1, SW_PROD_4.12
- removed net ADDR_BUS16: BANKA.48, BANKB.48, BANKC.48, SW_PROD_5.4
- removed net ADDR_BUS17: BANKA.17, BANKB.17, BANKC.17, SW_PROD_5.7
- removed net ADDR_BUS18: BANKA.16, BANKB.16, BANKC.16, SW_PROD_5.9
- removed net ADDR_BUS19: BANKA.9, BANKB.9, BANKC.9, SW_PROD_5.12
- removed net ADDR_BUS2: BANKA.23, BANKB.23, BANKC.23, SW_PROD_1.7
- removed net ADDR_BUS3: BANKA.22, BANKB.22, BANKC.22, SW_PROD_1.4
- removed net ADDR_BUS4: BANKA.21, BANKB.21, BANKC.21, SW_PROD_2.12
- removed net ADDR_BUS5: BANKA.20, BANKB.20, BANKC.20, SW_PROD_2.9
- removed net ADDR_BUS6: BANKA.19, BANKB.19, BANKC.19, SW_PROD_2.7
- removed net ADDR_BUS7: BANKA.18, BANKB.18, BANKC.18, SW_PROD_2.4
- removed net ADDR_BUS8: BANKA.8, BANKB.8, BANKC.8, SW_PROD_3.12
- removed net ADDR_BUS9: BANKA.7, BANKB.7, BANKC.7, SW_PROD_3.9
- removed net ADDR_SHIFT: ADD_LOW.1, ADD_LOW.2, JP3.5
- removed net BANKA_PROG: BANKA.11, JP4.5, R12.1
- removed net BANKB_PROG: BANKB.11, JP4.3, R13.1
- removed net BANKC_PROG: BANKC.11, JP4.1, R14.1
- removed net DATAA_SHIFT: BA_LOW.1, BA_LOW.2, JP3.6
- removed net DATAB_SHIFT: BB_LOW.1, BB_LOW.2, JP3.4
- removed net DATAC_SHIFT: BC_LOW.1, BC_LOW.2, JP3.3
- removed net DATA_ADDR_CLOCK: BA_HIGH.8, BA_LOW.8, BB_HIGH.8, BB_LOW.8, BC_HIGH.8, BC_LOW.8, JP3.7
- removed net N$37: BANKA.27, BANKA.46, BANKB.27, BANKB.46, BANKC.27, BANKC.46
- removed net N$42: BANKA.28, BANKB.28, BANKC.28, READ_WRITE.2
- removed net PROGRAM: JP3.9, JP4.2, JP4.4, JP4.6
- removed net PROG_ADDR0: ADD_LOW.3, SW_PROD_1.13
- removed net PROG_ADDR1: ADD_LOW.4, SW_PROD_1.10
- removed net PROG_ADDR10: ADD_MID.5, SW_PROD_3.6
- removed net PROG_ADDR11: ADD_MID.6, SW_PROD_3.3
- removed net PROG_ADDR12: ADD_MID.10, SW_PROD_4.3
- removed net PROG_ADDR13: ADD_MID.11, SW_PROD_4.6
- removed net PROG_ADDR14: ADD_MID.12, SW_PROD_4.10
- removed net PROG_ADDR15: ADD_HIGH.1, ADD_HIGH.2, ADD_MID.13, SW_PROD_4.13
- removed net PROG_ADDR16: ADD_HIGH.3, SW_PROD_5.3
- removed net PROG_ADDR17: ADD_HIGH.4, SW_PROD_5.6
- removed net PROG_ADDR18: ADD_HIGH.5, SW_PROD_5.10
- removed net PROG_ADDR19: ADD_HIGH.6, SW_PROD_5.13
- removed net PROG_ADDR2: ADD_LOW.5, SW_PROD_1.6
- removed net PROG_ADDR3: ADD_LOW.6, SW_PROD_1.3
- removed net PROG_ADDR4: ADD_LOW.10, SW_PROD_2.13
- removed net PROG_ADDR5: ADD_LOW.11, SW_PROD_2.10
- removed net PROG_ADDR6: ADD_LOW.12, SW_PROD_2.6
- removed net PROG_ADDR7: ADD_LOW.13, ADD_MID.1, ADD_MID.2, SW_PROD_2.3
- removed net PROG_ADDR8: ADD_MID.3, SW_PROD_3.13
- removed net PROG_ADDR9: ADD_MID.4, SW_PROD_3.10
- removed net PROG_ADDR_CLOCK: ADD_HIGH.8, ADD_LOW.8, ADD_MID.8, JP3.8
- removed net PROG_CLEAR: ADD_HIGH.9, ADD_LOW.9, ADD_MID.9, BA_HIGH.9, BA_LOW.9, BB_HIGH.9, BB_LOW.9, BC_HIGH.9, BC_LOW.9, JP3.10
- removed net PROG_DIR: JP3.1, SW_PROD_1.1, SW_PROD_2.1, SW_PROD_3.1, SW_PROD_4.1, SW_PROD_5.1
- removed net WRITE_ENABLE: BANKA.14, BANKB.14, BANKC.14, JP3.2
- net !CLEAR: no longer BANKA.12, BANKB.12, BANKC.12
- net DATAA0: now also BANKA.1; no longer BANKA.29, BA_LOW.3
- net DATAA1: now also BANKA.2; no longer BANKA.31, BA_LOW.4
- net DATAA10: now also BANKA.11; no longer BANKA.34, BA_HIGH.5
- net DATAA11: now also BANKA.12; no longer BANKA.36, BA_HIGH.6
- net DATAA12: now also BANKA.13; no longer BANKA.39, BA_HIGH.10
- net DATAA13: now also BANKA.14; no longer BANKA.41, BA_HIGH.11
- net DATAA14: now also BANKA.15; no longer BANKA.43, BA_HIGH.12
- net DATAA15: now also BANKA.16; no longer BANKA.45, BA_HIGH.13
- net DATAA2: now also BANKA.3; no longer BANKA.33, BA_LOW.5
- net DATAA3: now also BANKA.4; no longer BANKA.35, BA_LOW.6
- net DATAA4: now also BANKA.5; no longer BANKA.38, BA_LOW.10
- net DATAA5: now also BANKA.6; no longer BANKA.40, BA_LOW.11
- net DATAA6: now also BANKA.7; no longer BANKA.42, BA_LOW.12
- net DATAA7: now also BANKA.8; no longer BANKA.44, BA_HIGH.1, BA_HIGH.2, BA_LOW.13
- net DATAA8: now also BANKA.9; no longer BANKA.30, BA_HIGH.3
- net DATAA9: now also BANKA.10; no longer BANKA.32, BA_HIGH.4
- net DATAB0: now also BANKB.1; no longer BANKB.29, BB_LOW.3
- net DATAB1: now also BANKB.2; no longer BANKB.31, BB_LOW.4
- net DATAB10: now also BANKB.11; no longer BANKB.34, BB_HIGH.5
- net DATAB11: now also BANKB.12; no longer BANKB.36, BB_HIGH.6
- net DATAB12: now also BANKB.13; no longer BANKB.39, BB_HIGH.10
- net DATAB13: now also BANKB.14; no longer BANKB.41, BB_HIGH.11
- net DATAB14: now also BANKB.15; no longer BANKB.43, BB_HIGH.12
- net DATAB15: now also BANKB.16; no longer BANKB.45, BB_HIGH.13
- net DATAB2: now also BANKB.3; no longer BANKB.33, BB_LOW.5
- net DATAB3: now also BANKB.4; no longer BANKB.35, BB_LOW.6
- net DATAB4: now also BANKB.5; no longer BANKB.38, BB_LOW.10
- net DATAB5: now also BANKB.6; no longer BANKB.40, BB_LOW.11
- net DATAB6: now also BANKB.7; no longer BANKB.42, BB_LOW.12
- net DATAB7: now also BANKB.8; no longer BANKB.44, BB_HIGH.1, BB_HIGH.2, BB_LOW.13
- net DATAB8: now also BANKB.9; no longer BANKB.30, BB_HIGH.3
- net DATAB9: now also BANKB.10; no longer BANKB.32, BB_HIGH.4
- net DATAC0: now also BANKC.1; no longer BANKC.29, BC_LOW.3
- net DATAC1: now also BANKC.2; no longer BANKC.31, BC_LOW.4
- net DATAC10: now also BANKC.11; no longer BANKC.34, BC_HIGH.5
- net DATAC11: now also BANKC.12; no longer BANKC.36, BC_HIGH.6
- net DATAC12: now also BANKC.13; no longer BANKC.39, BC_HIGH.10
- net DATAC13: now also BANKC.14; no longer BANKC.41, BC_HIGH.11
- net DATAC14: now also BANKC.15; no longer BANKC.43, BC_HIGH.12
- net DATAC15: now also BANKC.16; no longer BANKC.45, BC_HIGH.13
- net DATAC2: now also BANKC.3; no longer BANKC.33, BC_LOW.5
- net DATAC3: now also BANKC.4; no longer BANKC.35, BC_LOW.6
- net DATAC4: now also BANKC.5; no longer BANKC.38, BC_LOW.10
- net DATAC5: now also BANKC.6; no longer BANKC.40, BC_LOW.11
- net DATAC6: now also BANKC.7; no longer BANKC.42, BC_LOW.12
- net DATAC7: now also BANKC.8; no longer BANKC.44, BC_HIGH.1, BC_HIGH.2, BC_LOW.13
- net DATAC8: now also BANKC.9; no longer BANKC.30, BC_HIGH.3
- net DATAC9: now also BANKC.10; no longer BANKC.32, BC_HIGH.4
- net GND: now also SV2.2, SV2.3; no longer ADD_HIGH.7, ADD_LOW.7, ADD_MID.7, BANKA.26, BANKA.37, BANKB.26, BANKB.37, BANKC.26, BANKC.37, BA_HIGH.7, BA_LOW.7, BB_HIGH.7, BB_LOW.7, BC_HIGH.7, BC_LOW.7, JP3.11, READ_WRITE.3, SW_PROD_1.15, SW_PROD_1.8, SW_PROD_2.15, SW_PROD_2.8, SW_PROD_3.15, SW_PROD_3.8, SW_PROD_4.15, SW_PROD_4.8, SW_PROD_5.15, SW_PROD_5.8
- net IN_BUS0: now also JP3.20; no longer SW_PROD_1.14
- net IN_BUS1: now also JP3.10; no longer SW_PROD_1.11
- net IN_BUS10: now also JP3.15; no longer SW_PROD_3.5
- net IN_BUS11: now also JP3.5; no longer SW_PROD_3.2
- net IN_BUS12: now also JP3.14; no longer SW_PROD_4.2
- net IN_BUS13: now also JP3.4; no longer SW_PROD_4.5
- net IN_BUS14: now also JP3.13; no longer SW_PROD_4.11
- net IN_BUS15: now also JP3.3; no longer SW_PROD_4.14
- net IN_BUS16: now also JP3.12; no longer SW_PROD_5.2
- net IN_BUS17: now also JP3.2; no longer SW_PROD_5.5
- net IN_BUS18: now also JP3.11; no longer SW_PROD_5.11
- net IN_BUS19: now also JP3.1; no longer SW_PROD_5.14
- net IN_BUS2: now also JP3.19; no longer SW_PROD_1.5
- net IN_BUS3: now also JP3.9; no longer SW_PROD_1.2
- net IN_BUS4: now also JP3.18; no longer SW_PROD_2.14
- net IN_BUS5: now also JP3.8; no longer SW_PROD_2.11
- net IN_BUS6: now also JP3.17; no longer SW_PROD_2.5
- net IN_BUS7: now also JP3.7; no longer SW_PROD_2.2
- net IN_BUS8: now also JP3.16; no longer SW_PROD_3.14
- net IN_BUS9: now also JP3.6; no longer SW_PROD_3.11
- net VCC: now also SV2.1, SV2.4, SV2.5, SV2.6; no longer ADD_HIGH.14, ADD_LOW.14, ADD_MID.14, BA_HIGH.14, BA_LOW.14, BB_HIGH.14, BB_LOW.14, BC_HIGH.14, BC_LOW.14, JP3.12, R12.2, R13.2, R14.2, READ_WRITE.1, SW_PROD_1.16, SW_PROD_2.16, SW_PROD_3.16, SW_PROD_4.16, SW_PROD_5.16
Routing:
- net PROG_CLEAR: track 269.6 -> 0.00 mm, vias 8 -> 0
- net DATA_ADDR_CLOCK: track 265.0 -> 0.00 mm, vias 9 -> 0
- net ADDR_SHIFT: track 210.1 -> 0.00 mm, vias 1 -> 0
- net GND: track 711.5 -> 506.9 mm, vias 25 -> 16
- net !CLEAR: track 263.6 -> 61.2 mm, vias 6 -> 1
- net VCC: track 820.8 -> 630.4 mm, vias 23 -> 26
- net PROG_ADDR_CLOCK: track 180.8 -> 0.00 mm, vias 3 -> 0
- net DATAA_SHIFT: track 175.7 -> 0.00 mm
- net N$61: track 233.1 -> 399.4 mm, vias 4 -> 8
- net ADDR_BUS12: track 162.6 -> 0.00 mm
- net ADDR_BUS1: track 157.2 -> 0.00 mm, vias 4 -> 0
- net DATAC_SHIFT: track 152.6 -> 0.00 mm, vias 4 -> 0
- net PROG_DIR: track 150.6 -> 0.00 mm, vias 6 -> 0
- net ADDR_BUS3: track 135.1 -> 0.00 mm, vias 4 -> 0
- net DATAC4: track 176.0 -> 41.0 mm, vias 4 -> 0
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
